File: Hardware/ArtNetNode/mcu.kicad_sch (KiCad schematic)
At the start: 1 part, among them U9 RP2040

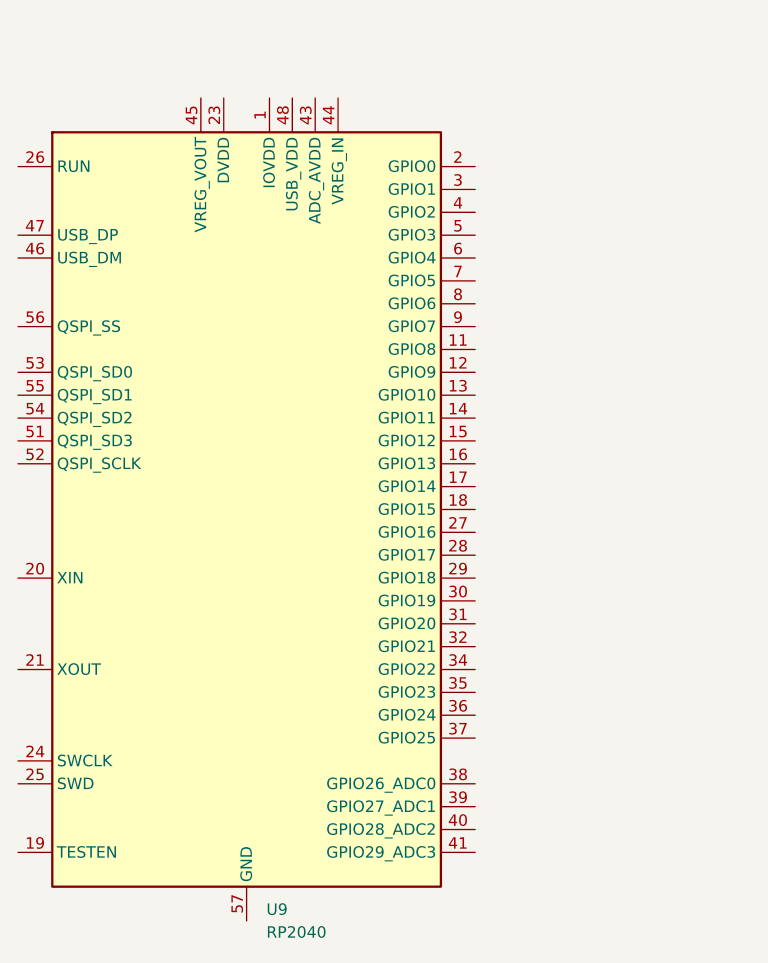
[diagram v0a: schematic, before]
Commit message: finished dmx interfaces
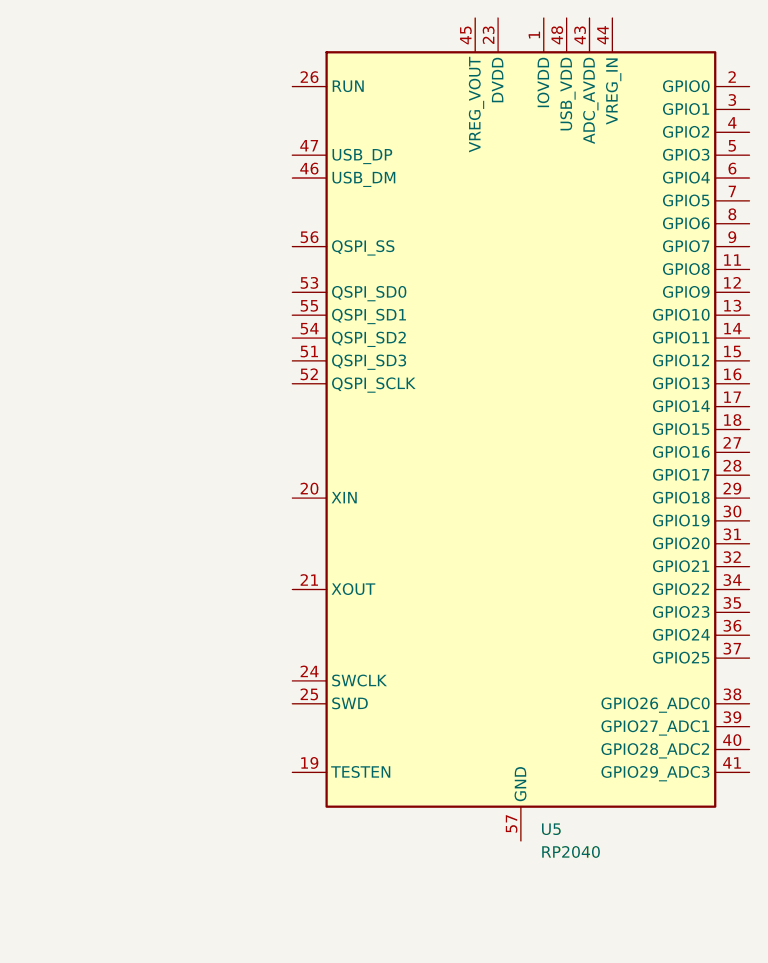
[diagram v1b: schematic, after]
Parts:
- renumbered U9 to U5
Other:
- moved on the sheet: U5
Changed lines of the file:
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@@
 	(symbol
 		(lib_id "MCU_RaspberryPi:RP2040")
-		(at 151.13 152.4 0)
+		(at 181.61 143.51 0)
 		(unit 1)
 		(exclude_from_sim no)
@@
 		(dnp no)
 		(fields_autoplaced yes)
-		(property "Reference" "U9"
-			(at 153.3241 196.85 0)
+		(property "Reference" "U5"
+			(at 183.8041 187.96 0)
 			(effects
 				(font
@@
 		)
 		(property "Value" "RP2040"
-			(at 153.3241 199.39 0)
+			(at 183.8041 190.5 0)
 			(effects
 				(font
@@
 		)
 		(property "Footprint" "Package_DFN_QFN:QFN-56-1EP_7x7mm_P0.4mm_EP3.2x3.2mm"
-			(at 151.13 152.4 0)
+			(at 181.61 143.51 0)
 			(effects
 				(font
@@
 		)
 		(property "Datasheet" "https://datasheets.raspberrypi.com/rp2040/rp2040-datasheet.pdf"
-			(at 151.13 152.4 0)
+			(at 181.61 143.51 0)
 			(effects
 				(font
@@
 		)
 		(property "Description" "A microcontroller by Raspberry Pi"
-			(at 151.13 152.4 0)
+			(at 181.61 143.51 0)
 			(effects
 				(font
@@
 			(project ""
 				(path "/5fe0a06d-00fb-4ef8-80af-4dd06c5496d9/efc89bbc-2463-427a-9fa7-bd6145ec8808"
-					(reference "U9")
+					(reference "U5")
 					(unit 1)
 				)
